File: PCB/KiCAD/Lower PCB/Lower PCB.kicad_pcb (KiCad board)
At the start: 2 copper layers, 179.5 x 163.2 mm, 0 parts

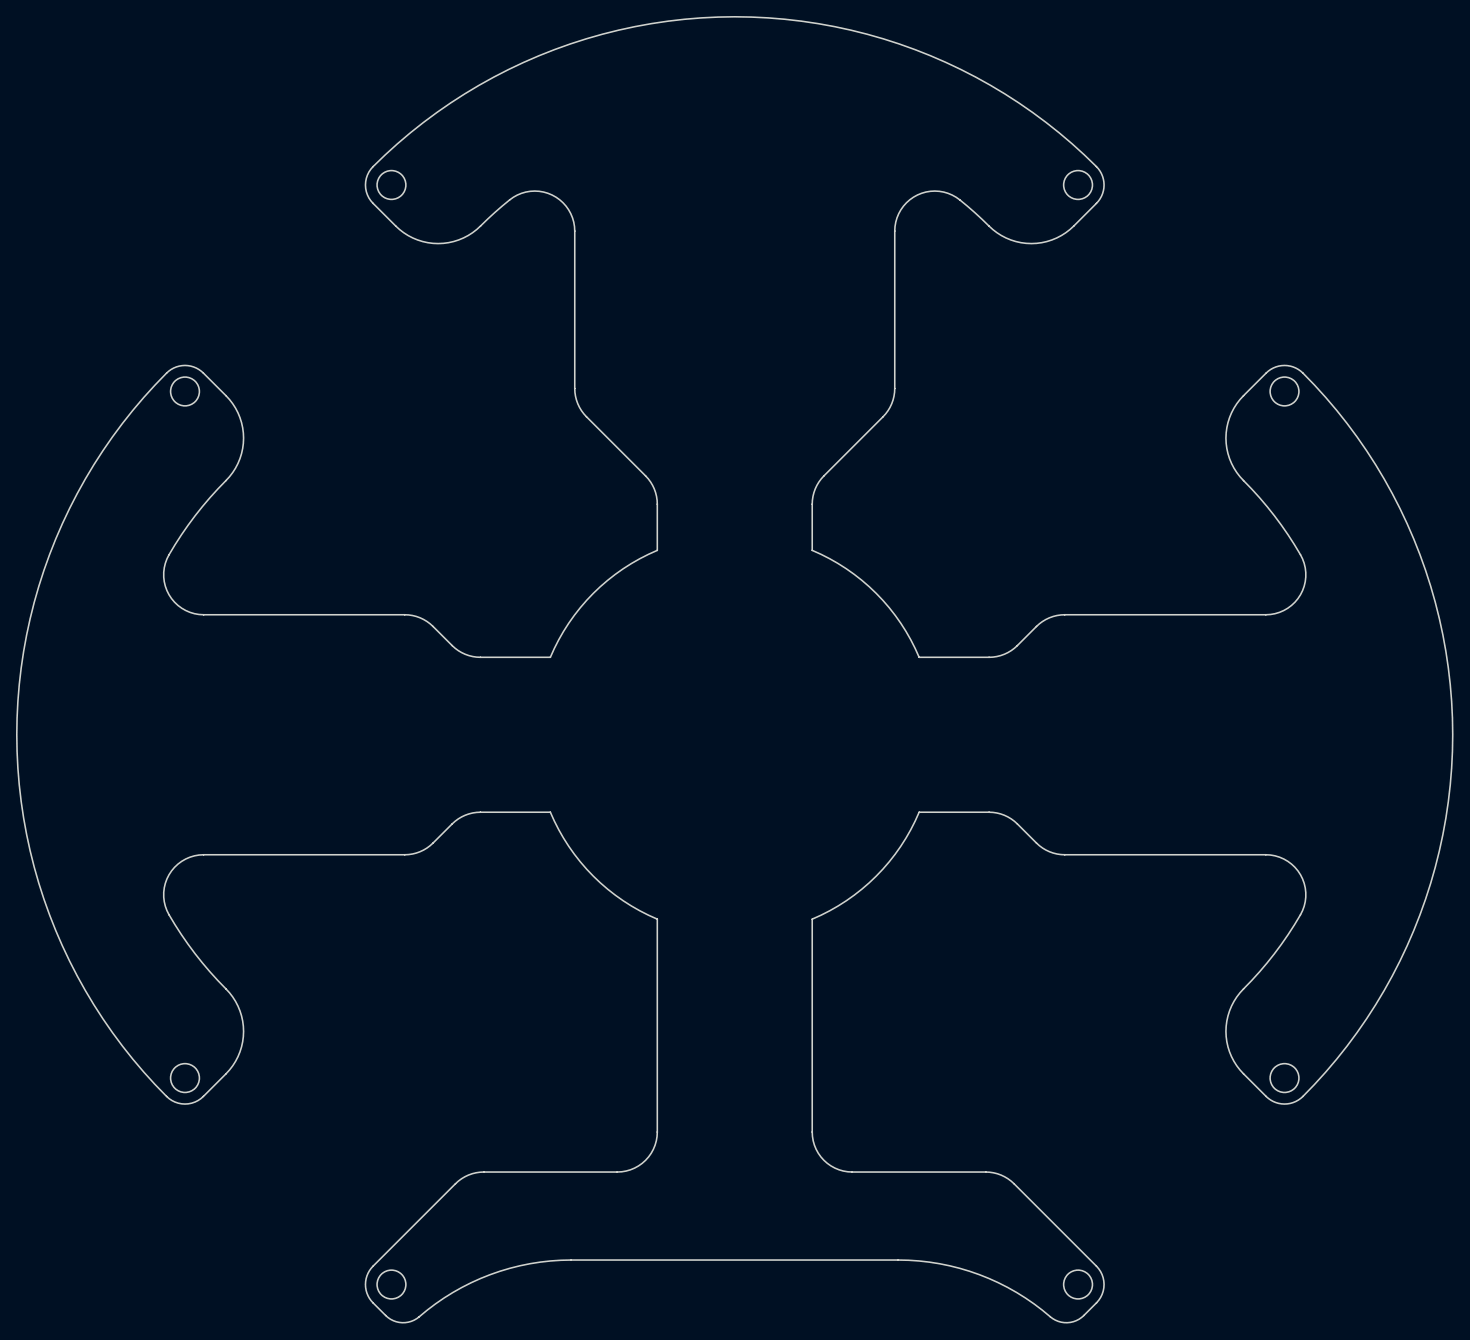
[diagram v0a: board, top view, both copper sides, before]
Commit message: Start of PCBs
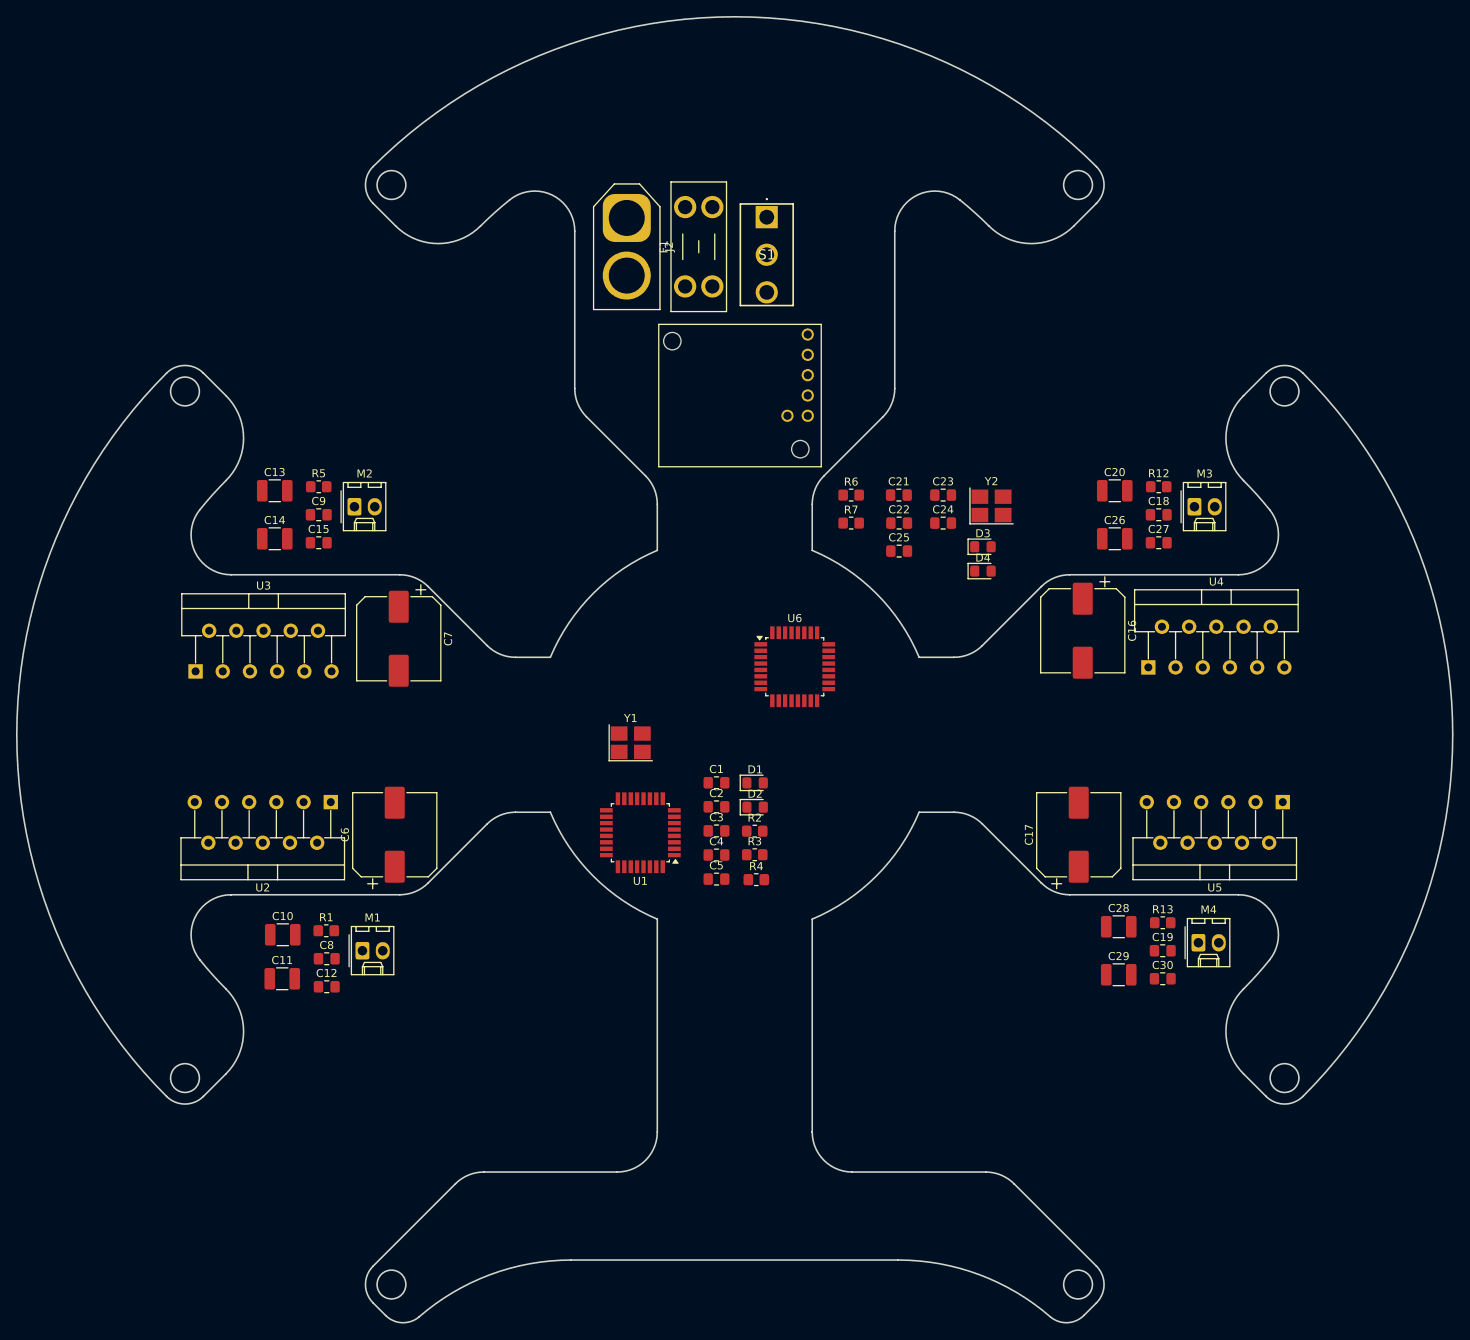
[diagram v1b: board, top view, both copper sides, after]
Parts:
- added C1: 100nF, Capacitor_SMD:C_0805_2012Metric_Pad1.18x1.45mm_HandSolder, F.Cu at (-2.28, 6.00)
- added C10: 10nF, Capacitor_SMD:C_1210_3225Metric_Pad1.33x2.70mm_HandSolder, F.Cu at (-56.5, 25.0)
- added C11: 10nF, Capacitor_SMD:C_1210_3225Metric_Pad1.33x2.70mm_HandSolder, F.Cu at (-56.6, 30.5)
- added C12: 0.1uF, Capacitor_SMD:C_0805_2012Metric_Pad1.18x1.45mm_HandSolder, F.Cu at (-51.0, 31.5)
- added C13: 10nF, Capacitor_SMD:C_1210_3225Metric_Pad1.33x2.70mm_HandSolder, F.Cu at (-57.5, -30.5)
- added C14: 10nF, Capacitor_SMD:C_1210_3225Metric_Pad1.33x2.70mm_HandSolder, F.Cu at (-57.5, -24.5)
- added C15: 0.1uF, Capacitor_SMD:C_0805_2012Metric_Pad1.18x1.45mm_HandSolder, F.Cu at (-52.0, -24.0)
- added C16: 220uF, Capacitor_SMD:CP_Elec_10x10, F.Cu at (43.5, -13.0)
- added C17: 220uF, Capacitor_SMD:CP_Elec_10x10, F.Cu at (43.0, 12.5)
- added C18: 0.1uF, Capacitor_SMD:C_0805_2012Metric_Pad1.18x1.45mm_HandSolder, F.Cu at (53.0, -27.5)
- added C19: 0.1uF, Capacitor_SMD:C_0805_2012Metric_Pad1.18x1.45mm_HandSolder, F.Cu at (53.5, 27.0)
- added C2: 100nF, Capacitor_SMD:C_0805_2012Metric_Pad1.18x1.45mm_HandSolder, F.Cu at (-2.28, 9.01)
- added C20: 10nF, Capacitor_SMD:C_1210_3225Metric_Pad1.33x2.70mm_HandSolder, F.Cu at (47.5, -30.5)
- added C21: 100nF, Capacitor_SMD:C_0805_2012Metric_Pad1.18x1.45mm_HandSolder, F.Cu at (20.5, -30.0)
- added C22: 100nF, Capacitor_SMD:C_0805_2012Metric_Pad1.18x1.45mm_HandSolder, F.Cu at (20.6, -26.5)
- added C23: 22pF, Capacitor_SMD:C_0805_2012Metric_Pad1.18x1.45mm_HandSolder, F.Cu at (26.1, -30.0)
- added C24: 22pF, Capacitor_SMD:C_0805_2012Metric_Pad1.18x1.45mm_HandSolder, F.Cu at (26.1, -26.5)
- added C25: 100nF, Capacitor_SMD:C_0805_2012Metric_Pad1.18x1.45mm_HandSolder, F.Cu at (20.6, -23.0)
- added C26: 10nF, Capacitor_SMD:C_1210_3225Metric_Pad1.33x2.70mm_HandSolder, F.Cu at (47.5, -24.5)
- added C27: 0.1uF, Capacitor_SMD:C_0805_2012Metric_Pad1.18x1.45mm_HandSolder, F.Cu at (53.0, -24.0)
- added C28: 10nF, Capacitor_SMD:C_1210_3225Metric_Pad1.33x2.70mm_HandSolder, F.Cu at (48.0, 24.0)
- added C29: 10nF, Capacitor_SMD:C_1210_3225Metric_Pad1.33x2.70mm_HandSolder, F.Cu at (48.0, 30.0)
- added C3: 100nF, Capacitor_SMD:C_0805_2012Metric_Pad1.18x1.45mm_HandSolder, F.Cu at (-2.28, 12.0)
- added C30: 0.1uF, Capacitor_SMD:C_0805_2012Metric_Pad1.18x1.45mm_HandSolder, F.Cu at (53.5, 30.5)
- added C4: 22pF, Capacitor_SMD:C_0805_2012Metric_Pad1.18x1.45mm_HandSolder, F.Cu at (-2.28, 15.0)
- added C5: 22pF, Capacitor_SMD:C_0805_2012Metric_Pad1.18x1.45mm_HandSolder, F.Cu at (-2.28, 18.0)
- added C6: 220uF, Capacitor_SMD:CP_Elec_10x10, F.Cu at (-42.5, 12.5)
- added C7: 220uF, Capacitor_SMD:CP_Elec_10x10, F.Cu at (-42.0, -12.0)
- added C8: 0.1uF, Capacitor_SMD:C_0805_2012Metric_Pad1.18x1.45mm_HandSolder, F.Cu at (-51.0, 28.0)
- added C9: 0.1uF, Capacitor_SMD:C_0805_2012Metric_Pad1.18x1.45mm_HandSolder, F.Cu at (-52.0, -27.5)
- added D1: RED_LED, LED_SMD:LED_0805_2012Metric_Pad1.15x1.40mm_HandSolder, F.Cu at (2.54, 6.01)
- added D2: GREEN_LED, LED_SMD:LED_0805_2012Metric_Pad1.15x1.40mm_HandSolder, F.Cu at (2.54, 9.05)
- added D3: RED_LED, LED_SMD:LED_0805_2012Metric_Pad1.15x1.40mm_HandSolder, F.Cu at (31.0, -23.5)
- added D4: GREEN_LED, LED_SMD:LED_0805_2012Metric_Pad1.15x1.40mm_HandSolder, F.Cu at (31.0, -20.5)
- added F1: Fuse, Fuse:Fuseholder_Blade_Mini_Keystone_3568, F.Cu at (-6.20, -56.0)
- added J2: Conn_01x02, Connector_AMASS:AMASS_XT60-M_1x02_P7.20mm_Vertical, F.Cu at (-13.5, -64.6)
- added M1: Conn_01x02_Pin, Connector_Molex:Molex_KK-254_AE-6410-02A_1x02_P2.54mm_Vertical, F.Cu at (-46.5, 27.0)
- added M2: Conn_01x02_Pin, Connector_Molex:Molex_KK-254_AE-6410-02A_1x02_P2.54mm_Vertical, F.Cu at (-47.5, -28.5)
- added M3: Conn_01x02_Pin, Connector_Molex:Molex_KK-254_AE-6410-02A_1x02_P2.54mm_Vertical, F.Cu at (57.5, -28.5)
- added M4: Conn_01x02_Pin, Connector_Molex:Molex_KK-254_AE-6410-02A_1x02_P2.54mm_Vertical, F.Cu at (58.0, 26.0)
- added R1: 2.7k, Resistor_SMD:R_0805_2012Metric_Pad1.20x1.40mm_HandSolder, F.Cu at (-51.1, 24.5)
- added R12: 2.7k, Resistor_SMD:R_0805_2012Metric_Pad1.20x1.40mm_HandSolder, F.Cu at (53.0, -31.0)
- added R13: 2.7k, Resistor_SMD:R_0805_2012Metric_Pad1.20x1.40mm_HandSolder, F.Cu at (53.5, 23.5)
- added R2: 330, Resistor_SMD:R_0805_2012Metric_Pad1.20x1.40mm_HandSolder, F.Cu at (2.50, 12.1)
- added R3: 330, Resistor_SMD:R_0805_2012Metric_Pad1.20x1.40mm_HandSolder, F.Cu at (2.50, 15.0)
- added R4: 330, Resistor_SMD:R_0805_2012Metric_Pad1.20x1.40mm_HandSolder, F.Cu at (2.69, 18.1)
- added R5: 2.7k, Resistor_SMD:R_0805_2012Metric_Pad1.20x1.40mm_HandSolder, F.Cu at (-52.0, -31.0)
- added R6: 330, Resistor_SMD:R_0805_2012Metric_Pad1.20x1.40mm_HandSolder, F.Cu at (14.6, -30.0)
- added R7: 330, Resistor_SMD:R_0805_2012Metric_Pad1.20x1.40mm_HandSolder, F.Cu at (14.6, -26.5)
- added S1: 1101M2S3CGE2, 1101M2S3CGE2:1101M2S3CGE2, F.Cu at (4.00, -64.7)
- added U1: ATmega328PB-A, Package_QFP:TQFP-32_7x7mm_P0.8mm, F.Cu at (-11.8, 12.2)
- added U2: LMD18200, Package_TO_SOT_THT:TO-220-11_P3.4x5.08mm_StaggerOdd_Lead4.58mm_Vertical, F.Cu at (-50.5, 8.42)
- added U3: LMD18200, Package_TO_SOT_THT:TO-220-11_P3.4x5.08mm_StaggerOdd_Lead4.58mm_Vertical, F.Cu at (-67.4, -7.92)
- added U4: LMD18200, Package_TO_SOT_THT:TO-220-11_P3.4x5.08mm_StaggerOdd_Lead4.58mm_Vertical, F.Cu at (51.7, -8.42)
- added U5: LMD18200, Package_TO_SOT_THT:TO-220-11_P3.4x5.08mm_StaggerOdd_Lead4.58mm_Vertical, F.Cu at (68.5, 8.42)
- added U6: ATmega328PB-A, Package_QFP:TQFP-32_7x7mm_P0.8mm, F.Cu at (7.50, -8.50)
- added U7: ~, Pololu:D36V28F5, F.Cu at (0.00, -42.5)
- added Y1: Crystal, Crystal:Crystal_SMD_3225-4Pin_3.2x2.5mm_HandSoldering, F.Cu at (-13.0, 1.00)
- added Y2: Crystal, Crystal:Crystal_SMD_3225-4Pin_3.2x2.5mm_HandSoldering, F.Cu at (32.1, -28.6)
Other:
- outline, holes or cut-outs redrawn
